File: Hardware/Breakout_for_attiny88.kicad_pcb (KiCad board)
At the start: 2 copper layers, 22.9 x 48.5 mm, 12 parts, among them J1 HEADER, J2 HEADER, J3 AVR-ISP-6, J4 PWR, SW1 SW, U1 ATtiny88

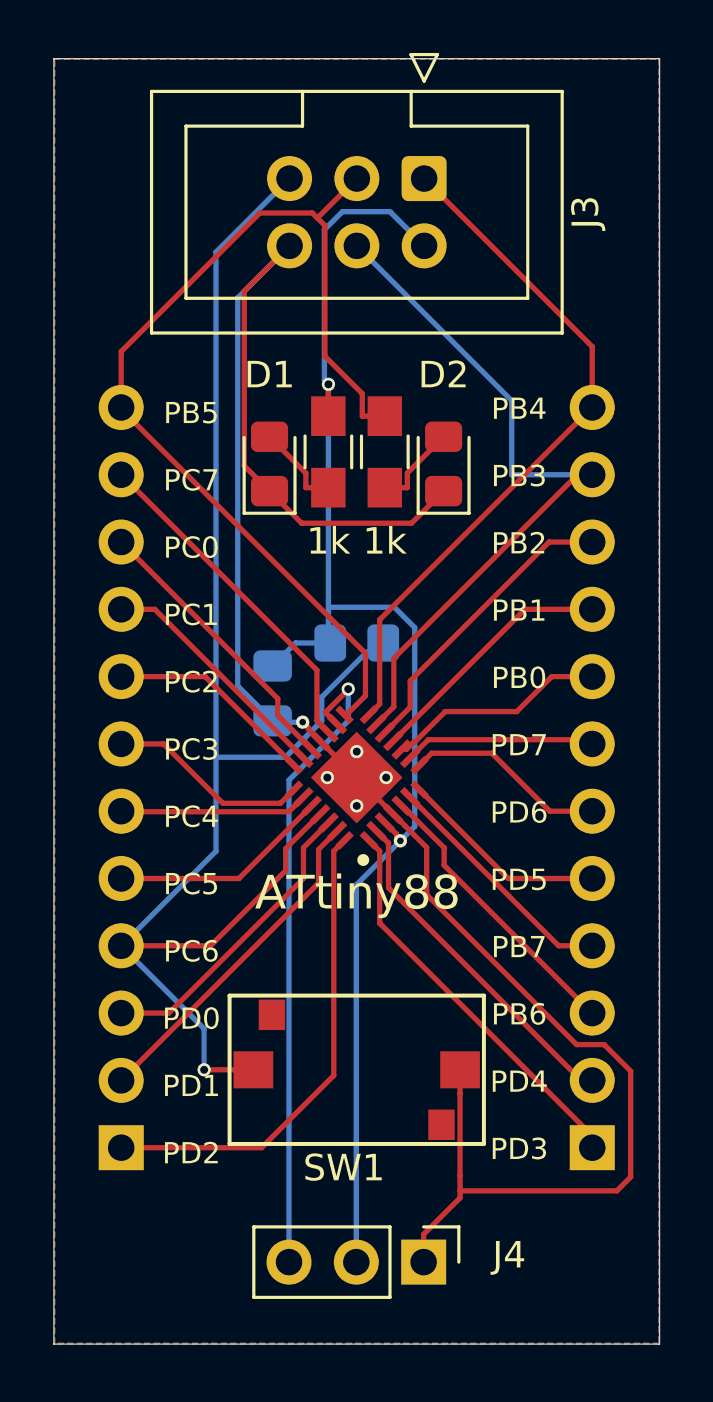
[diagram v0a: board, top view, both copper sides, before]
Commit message: Added_New_PCB
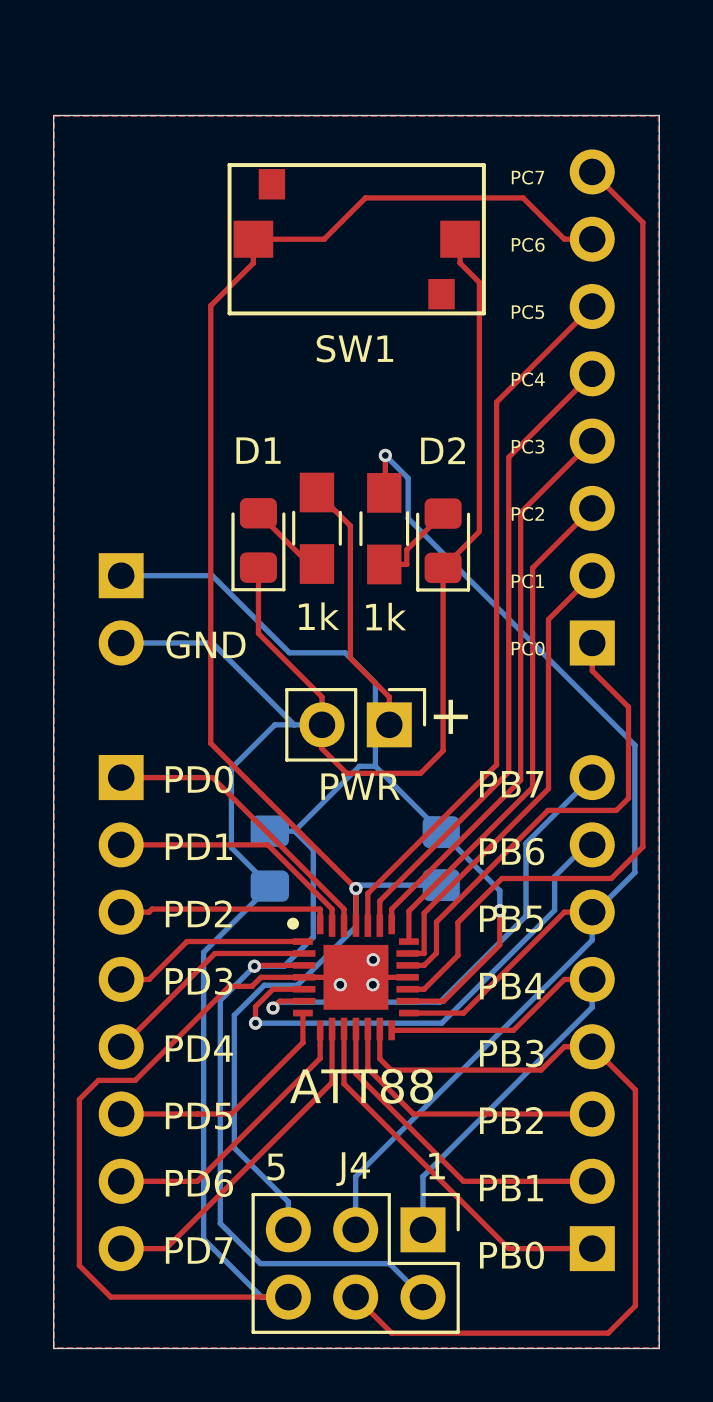
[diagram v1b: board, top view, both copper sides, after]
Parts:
- added J5: Conn_01x02, Connector_PinHeader_2.54mm:PinHeader_1x02_P2.54mm_Vertical, B.Cu at (139.6, 97.4)
- added J6: Conn_01x02, Connector_PinHeader_2.54mm:PinHeader_1x02_P2.54mm_Vertical, F.Cu at (149.7, 103.0)
- J1, J2: value HEADER -> Conn_01x08; footprint Pin_Headers:Pin_Header_Straight_1x12_Pitch2.54mm -> Connector_PinHeader_2.54mm:PinHeader_1x08_P2.54mm_Vertical
- J3: value AVR-ISP-6 -> Conn_01x08; footprint Connector_IDC:IDC-Header_2x03_P2.54mm_Vertical -> Connector_PinHeader_2.54mm:PinHeader_1x08_P2.54mm_Vertical; moved to B.Cu
- J4: value PWR -> AVR-ISP-6; footprint Pin_Headers:Pin_Header_Straight_1x03_Pitch2.54mm -> Connector_PinHeader_2.54mm:PinHeader_2x03_P2.54mm_Vertical
- SW1: footprint rhydo_labz_switch:rhydolabz_push_button_switch -> rest_switch:push_button_switch
- U1: value ATtiny88 -> ATT88
- moved SW1 31.3 mm to (148.5, 84.7)
- moved J2 26.1 mm to (157.4, 99.9)
- moved J3 25.3 mm to (139.6, 105.0), turned to 180 degrees
- moved R1 8.74 mm to (151.7, 108.1), turned to -90 degrees
- moved U1 7.54 mm to (148.5, 112.5), turned to 0 degrees
- moved C1 6.24 mm to (145.2, 108.1)
- moved J1 3.81 mm to (157.4, 122.8)
- moved D1 2.92 mm to (144.8, 96.0)
- moved R2 2.91 mm to (147.0, 95.6)
- moved D2 2.90 mm to (151.8, 96.1)
- moved R3 2.90 mm to (149.5, 95.6)
- moved J4 1.22 mm to (151.0, 122.1)
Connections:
- J1 pad 1: PD3 -> PB0
- J1 pad 2: PD4 -> PB1
- J1 pad 3: PB6 -> PB2
- J1 pad 4: PB7 -> MOSI
- J1 pad 5: PD5 -> MISO
- J1 pad 6: PD6 -> PB5
- J1 pad 7: PD7 -> PB6
- J1 pad 8: PB0 -> PB7
- J2 pad 1: PD2 -> PC0
- J2 pad 2: PD1 -> PC1
- J2 pad 3: PD0 -> PC2
- J2 pad 4: PC6 -> PC3
- J2 pad 5: PC5 -> PC4
- J2 pad 6: PC4 -> PC5
- J2 pad 7: PC3 -> PC6
- J2 pad 8: PC2 -> PC7
- J3 pad 1: MISO -> PD0
- J3 pad 2: VCC -> PD1
- J3 pad 3: SCK -> PD2
- J3 pad 4: MOSI -> PD3
- J3 pad 5: PC6 -> PD4
- J3 pad 6: GND -> PD5
- J4 pad 1: GND -> MISO
- J4 pad 3: AVCC -> PB5
- R3 pad 1: SCK -> PB5
- SW1 pad 3: GND -> (no net)
- U1 pad 15: SCK -> PB5
- U1 pad 16: AVCC -> VCC
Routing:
- net PB5: track 0.00 -> 47.5 mm, vias 0 -> 1
- net SCK: track 38.7 -> 0.00 mm
- net PC7: track 13.0 -> 38.1 mm
- net AVCC: track 24.4 -> 0.00 mm, vias 1 -> 0
- net GND: track 75.8 -> 97.7 mm, vias 5 -> 3
- net PC5: track 8.33 -> 26.9 mm
- net PC4: track 7.11 -> 24.2 mm
- net VCC: track 53.9 -> 70.8 mm
- net PC3: track 7.71 -> 21.4 mm
- net PC2: track 7.96 -> 19.2 mm
- net PD2: track 18.2 -> 8.13 mm
- net PB7: track 9.20 -> 18.6 mm, vias 0 -> 1
- net PC1: track 9.20 -> 17.5 mm
- net PB6: track 10.8 -> 19.0 mm, vias 0 -> 1
- net PD3: track 15.1 -> 7.45 mm
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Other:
- board size 22.9 x 48.5 mm -> 22.9 x 46.5 mm
- board text added: "+"
- board text added: "1"
- board text added: "5"
- board text added: "GND"
